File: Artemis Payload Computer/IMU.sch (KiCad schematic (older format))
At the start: 1 part

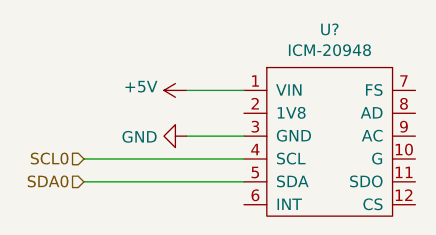
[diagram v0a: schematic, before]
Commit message: Continued work on SD card. Starting PCB layout.
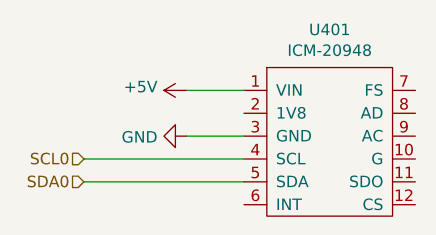
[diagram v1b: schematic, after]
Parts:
- gave numbers to parts that had none: 1
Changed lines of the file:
@@
 $EndDescr
 $Comp
-L Artemis_Footprints:ICM-20948 U?
+L Artemis_Footprints:ICM-20948 U401
 U 1 1 60405DA7
 P 6200 3000
-F 0 "U?" H 6225 3165 50  0000 C CNN
+F 0 "U401" H 6225 3165 50  0000 C CNN
 F 1 "ICM-20948" H 6225 3074 50  0000 C CNN
 F 2 "Artemis Payload Computer:ICM-20948" H 6200 3000 50  0001 C CNN
@@
 $EndComp
 $Comp
-L power:+5V #PWR?
+L power:+5V #PWR0109
 U 1 1 604076E6
 P 5600 3100
-F 0 "#PWR?" H 5600 2950 50  0001 C CNN
+F 0 "#PWR0109" H 5600 2950 50  0001 C CNN
 F 1 "+5V" V 5615 3228 50  0000 L CNN
 F 2 "" H 5600 3100 50  0001 C CNN
@@
 $EndComp
 $Comp
-L power:GND #PWR?
+L power:GND #PWR0110
 U 1 1 604079B0
 P 5600 3300
-F 0 "#PWR?" H 5600 3050 50  0001 C CNN
+F 0 "#PWR0110" H 5600 3050 50  0001 C CNN
 F 1 "GND" V 5605 3172 50  0000 R CNN
 F 2 "" H 5600 3300 50  0001 C CNN
